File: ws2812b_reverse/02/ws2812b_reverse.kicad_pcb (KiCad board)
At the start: 2 copper layers, 10.2 x 10.5 mm, 4 parts, among them J1 CONN_01X04, J2 CONN_01X04

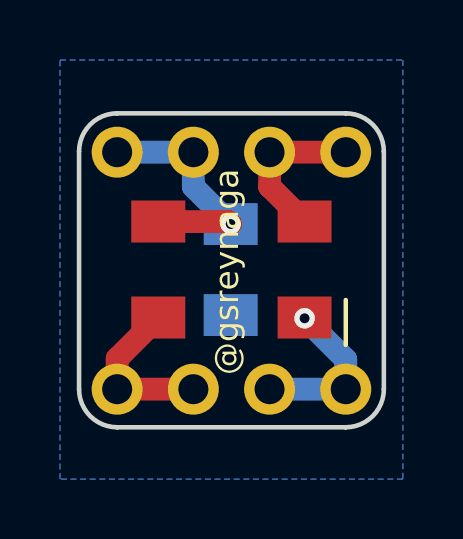
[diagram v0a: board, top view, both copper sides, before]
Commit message: Update
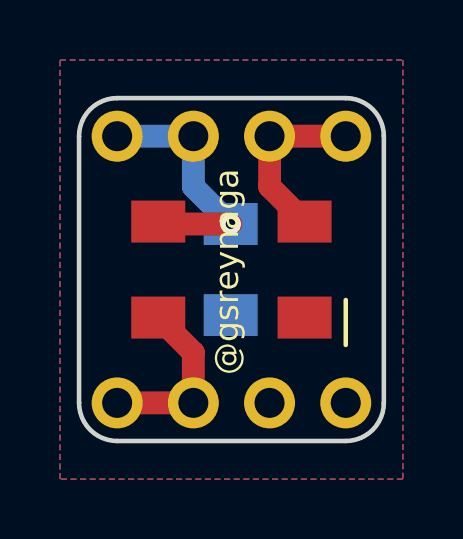
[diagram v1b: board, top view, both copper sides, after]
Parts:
- moved J1 0.53 mm to (-3.81, -3.81)
- moved J2 0.46 mm to (-3.81, 5.08)
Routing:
- net GND: track 5.47 -> 0.00 mm, vias 1 -> 0
- net Net-(J1-Pad3): track 5.56 -> 6.10 mm
- net VCC: track 7.90 -> 8.43 mm
- added copper zone on F.Cu, net GND
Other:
- board size 10.2 x 10.5 mm -> 10.2 x 11.4 mm
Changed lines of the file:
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@@
-(kicad_pcb (version 20171130) (host pcbnew 6.0.0-rc1-unknown-efe880b~66~ubuntu18.04.1)
+(kicad_pcb (version 20171130) (host pcbnew 6.0.0-rc1-unknown-ebdc383~66~ubuntu16.04.1)
   (general
     (thickness 1.6)
     (drawings 35)
-    (tracks 19)
+    (tracks 15)
     (zones 0)
     (modules 4)
@@
   )
   (setup
-    (last_trace_width 0.254)
+    (last_trace_width 0.762)
     (user_trace_width 0.1524)
     (user_trace_width 0.254)
@@
   )
   (module Connector_PinSocket_2.54mm:PinSocket_1x04_P2.54mm_WeMos (layer F.Cu)
-    (at -3.81 -3.2766 90)
+    (at -3.81 -3.81 90)
     (descr "Through hole straight socket strip, 1x04, 2.54mm pitch, single row (from Kicad 4.0.7), script generated")
     (tags "Through hole socket strip THT 1x04 2.54mm single row")
@@
   )
   (module Connector_PinSocket_2.54mm:PinSocket_1x04_P2.54mm_WeMos (layer F.Cu)
-    (at -3.81 4.6228 90)
+    (at -3.81 5.08 90)
     (descr "Through hole straight socket strip, 1x04, 2.54mm pitch, single row (from Kicad 4.0.7), script generated")
     (tags "Through hole socket strip THT 1x04 2.54mm single row")
@@
       (net 2 GND))
   )
-  (dimension 7.8994 (width 0.1524) (layer F.SilkS)
-    (gr_text "7.899 mm" (at -9.271 0.6731 90) (layer F.SilkS)
+  (dimension 8.89 (width 0.1524) (layer F.SilkS)
+    (gr_text "8.890 mm" (at 9.5758 0.635 270) (layer F.SilkS)
       (effects (font (size 1.016 1.016) (thickness 0.1524)))
     )
-    (feature1 (pts (xy -1.27 -3.2766) (xy -8.536621 -3.2766)))
-    (feature2 (pts (xy -1.27 4.6228) (xy -8.536621 4.6228)))
-    (crossbar (pts (xy -7.9502 4.6228) (xy -7.9502 -3.2766)))
-    (arrow1a (pts (xy -7.9502 -3.2766) (xy -7.363779 -2.150096)))
-    (arrow1b (pts (xy -7.9502 -3.2766) (xy -8.536621 -2.150096)))
-    (arrow2a (pts (xy -7.9502 4.6228) (xy -7.363779 3.496296)))
-    (arrow2b (pts (xy -7.9502 4.6228) (xy -8.536621 3.496296)))
+    (feature1 (pts (xy 3.81 5.08) (xy 8.841421 5.08)))
+    (feature2 (pts (xy 3.81 -3.81) (xy 8.841421 -3.81)))
+    (crossbar (pts (xy 8.255 -3.81) (xy 8.255 5.08)))
+    (arrow1a (pts (xy 8.255 5.08) (xy 7.668579 3.953496)))
+    (arrow1b (pts (xy 8.255 5.08) (xy 8.841421 3.953496)))
+    (arrow2a (pts (xy 8.255 -3.81) (xy 7.668579 -2.683496)))
+    (arrow2b (pts (xy 8.255 -3.81) (xy 8.841421 -2.683496)))
+  )
+  (dimension 11.43 (width 0.1524) (layer F.SilkS)
+    (gr_text "11.430 mm" (at -9.5758 0.635 270) (layer F.SilkS)
+      (effects (font (size 1.016 1.016) (thickness 0.1524)))
+    )
+    (feature1 (pts (xy -3.81 6.35) (xy -8.841421 6.35)))
+    (feature2 (pts (xy -3.81 -5.08) (xy -8.841421 -5.08)))
+    (crossbar (pts (xy -8.255 -5.08) (xy -8.255 6.35)))
+    (arrow1a (pts (xy -8.255 6.35) (xy -8.841421 5.223496)))
+    (arrow1b (pts (xy -8.255 6.35) (xy -7.668579 5.223496)))
+    (arrow2a (pts (xy -8.255 -5.08) (xy -8.841421 -3.953496)))
+    (arrow2b (pts (xy -8.255 -5.08) (xy -7.668579 -3.953496)))
   )
   (dimension 10.16 (width 0.1524) (layer F.SilkS)
@@
     (arrow2b (pts (xy 5.08 -10.16) (xy 3.953496 -9.573579)))
   )
-  (dimension 10.4648 (width 0.1524) (layer F.SilkS)
-    (gr_text "10.465 mm" (at 10.8458 0.6604 90) (layer F.SilkS)
-      (effects (font (size 1.016 1.016) (thickness 0.1524)))
-    )
-    (feature1 (pts (xy 3.81 -4.572) (xy 10.111421 -4.572)))
-    (feature2 (pts (xy 3.81 5.8928) (xy 10.111421 5.8928)))
-    (crossbar (pts (xy 9.525 5.8928) (xy 9.525 -4.572)))
-    (arrow1a (pts (xy 9.525 -4.572) (xy 10.111421 -3.445496)))
-    (arrow1b (pts (xy 9.525 -4.572) (xy 8.938579 -3.445496)))
-    (arrow2a (pts (xy 9.525 5.8928) (xy 10.111421 4.766296)))
-    (arrow2b (pts (xy 9.525 5.8928) (xy 8.938579 4.766296)))
-  )
   (gr_text @gsreynaga (at -0.1524 0.7112 90) (layer F.SilkS)
     (effects (font (size 0.8 0.8) (thickness 0.1524)))
@@
     (effects (font (size 1.016 1.016) (thickness 0.2)) (justify mirror))
   )
-  (gr_arc (start 3.81 4.6228) (end 3.81 5.8928) (angle -90) (layer Edge.Cuts) (width 0.1524))
-  (gr_arc (start -3.81 4.6228) (end -5.08 4.6228) (angle -90) (layer Edge.Cuts) (width 0.1524))
-  (gr_arc (start -3.81 -3.302) (end -3.81 -4.572) (angle -90) (layer Edge.Cuts) (width 0.1524))
-  (gr_arc (start 3.81 -3.302) (end 5.08 -3.302) (angle -90) (layer Edge.Cuts) (width 0.1524))
-  (gr_line (start 5.08 4.6228) (end 5.08 -3.302) (layer Edge.Cuts) (width 0.1524))
-  (gr_line (start -3.81 5.8928) (end 3.81 5.8928) (layer Edge.Cuts) (width 0.1524))
-  (gr_line (start -5.08 -3.302) (end -5.08 4.6228) (layer Edge.Cuts) (width 0.1524))
-  (gr_line (start 3.81 -4.572) (end -3.81 -4.572) (layer Edge.Cuts) (width 0.1524))
+  (gr_arc (start 3.81 5.08) (end 3.81 6.35) (angle -90) (layer Edge.Cuts) (width 0.1524))
+  (gr_arc (start -3.81 5.08) (end -5.08 5.08) (angle -90) (layer Edge.Cuts) (width 0.1524))
+  (gr_arc (start -3.81 -3.81) (end -3.81 -5.08) (angle -90) (layer Edge.Cuts) (width 0.1524))
+  (gr_arc (start 3.81 -3.81) (end 5.08 -3.81) (angle -90) (layer Edge.Cuts) (width 0.1524))
+  (gr_line (start 5.08 5.08) (end 5.08 -3.81) (layer Edge.Cuts) (width 0.1524))
+  (gr_line (start -3.81 6.35) (end 3.81 6.35) (layer Edge.Cuts) (width 0.1524))
+  (gr_line (start -5.08 -3.81) (end -5.08 5.08) (layer Edge.Cuts) (width 0.1524))
+  (gr_line (start 3.81 -5.08) (end -3.81 -5.08) (layer Edge.Cuts) (width 0.1524))
   (gr_circle (center 117.348 76.962) (end 118.618 76.962) (layer Dwgs.User) (width 0.15))
   (gr_line (start 114.427 78.994) (end 114.427 74.93) (angle 90) (layer Dwgs.User) (width 0.15))
@@
   (gr_line (start 104.648 82.55) (end 120.523 82.55) (angle 90) (layer Dwgs.User) (width 0.15))
   (via (at -0.0254 -0.8825) (size 0.6858) (drill 0.3302) (layers F.Cu B.Cu) (net 1))
-  (segment (start -0.1079 -0.965) (end -0.0254 -0.8825) (width 0.762) (layer F.Cu) (net 1))
-  (segment (start -2.4384 -0.965) (end -0.1079 -0.965) (width 0.762) (layer F.Cu) (net 1))
+  (segment (start -3.81 -3.81) (end -1.27 -3.81) (width 0.762) (layer B.Cu) (net 1))
   (segment (start -1.27 -2.1271) (end -0.0254 -0.8825) (width 0.762) (layer B.Cu) (net 1))
-  (segment (start -1.27 -3.2766) (end -1.27 -2.1271) (width 0.762) (layer B.Cu) (net 1))
-  (segment (start -3.81 -3.2766) (end -1.27 -3.2766) (width 0.762) (layer B.Cu) (net 1))
-  (via (at 2.4384 2.2606) (size 0.6858) (drill 0.3302) (layers F.Cu B.Cu) (net 2))
-  (segment (start 3.81 3.6322) (end 2.4384 2.2606) (width 0.762) (layer B.Cu) (net 2))
-  (segment (start 3.81 4.6228) (end 3.81 3.6322) (width 0.762) (layer B.Cu) (net 2))
-  (segment (start 1.27 4.6228) (end 3.81 4.6228) (width 0.762) (layer B.Cu) (net 2))
+  (segment (start -1.27 -3.81) (end -1.27 -2.1271) (width 0.762) (layer B.Cu) (net 1))
+  (segment (start -2.3559 -0.8825) (end -2.4384 -0.965) (width 0.762) (layer F.Cu) (net 1))
+  (segment (start -0.0254 -0.8825) (end -2.3559 -0.8825) (width 0.762) (layer F.Cu) (net 1))
   (segment (start -2.4384 2.235) (end -2.4384 2.2352) (width 0.762) (layer F.Cu) (net 3))
-  (segment (start -3.81 3.6066) (end -2.4384 2.235) (width 0.762) (layer F.Cu) (net 3))
-  (segment (start -3.81 4.6228) (end -3.81 3.6066) (width 0.762) (layer F.Cu) (net 3))
-  (segment (start -3.81 4.6228) (end -1.27 4.6228) (width 0.762) (layer F.Cu) (net 3))
+  (segment (start -3.81 5.08) (end -1.27 5.08) (width 0.762) (layer F.Cu) (net 3))
+  (segment (start -1.27 3.4034) (end -2.4384 2.235) (width 0.762) (layer F.Cu) (net 3))
+  (segment (start -1.27 5.08) (end -1.27 3.4034) (width 0.762) (layer F.Cu) (net 3))
   (segment (start 2.4384 -0.965) (end 2.21 -0.965) (width 0.762) (layer F.Cu) (net 4))
   (segment (start 2.4384 -0.965) (end 2.4384 -0.9652) (width 0.762) (layer F.Cu) (net 4))
+  (segment (start 3.81 -3.81) (end 1.27 -3.81) (width 0.762) (layer F.Cu) (net 4))
   (segment (start 1.27 -2.1334) (end 2.4384 -0.965) (width 0.762) (layer F.Cu) (net 4))
-  (segment (start 1.27 -3.2766) (end 1.27 -2.1334) (width 0.762) (layer F.Cu) (net 4))
-  (segment (start 1.27 -3.2766) (end 3.81 -3.2766) (width 0.762) (layer F.Cu) (net 4))
+  (segment (start 1.27 -3.81) (end 1.27 -2.1334) (width 0.762) (layer F.Cu) (net 4))
   (zone (net 2) (net_name GND) (layer B.Cu) (hatch edge 0.508)
     (connect_pads (clearance 0.508))
@@
     (polygon
       (pts
+        (xy -5.715 -6.35) (xy 5.715 -6.35) (xy 5.715 7.62) (xy -5.715 7.62)
+      )
+    )
+  )
+  (zone (net 2) (net_name GND) (layer F.Cu) (hatch edge 0.508)
+    (connect_pads (clearance 0.508))
+    (min_thickness 0.254)
+    (fill yes (arc_segments 32) (thermal_gap 0.508) (thermal_bridge_width 0.508))
+    (polygon
+      (pts
